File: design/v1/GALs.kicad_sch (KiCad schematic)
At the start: 19 parts, among them IC2 ATF22V10C, IC3 ATF22V10C, IC5 ATF22V10C, IC6 ATF22V10C, IC7 74LS148, IC8 ATF16V8BQL, J9 Conn_02x05_Odd_Even, U5 ATF1504

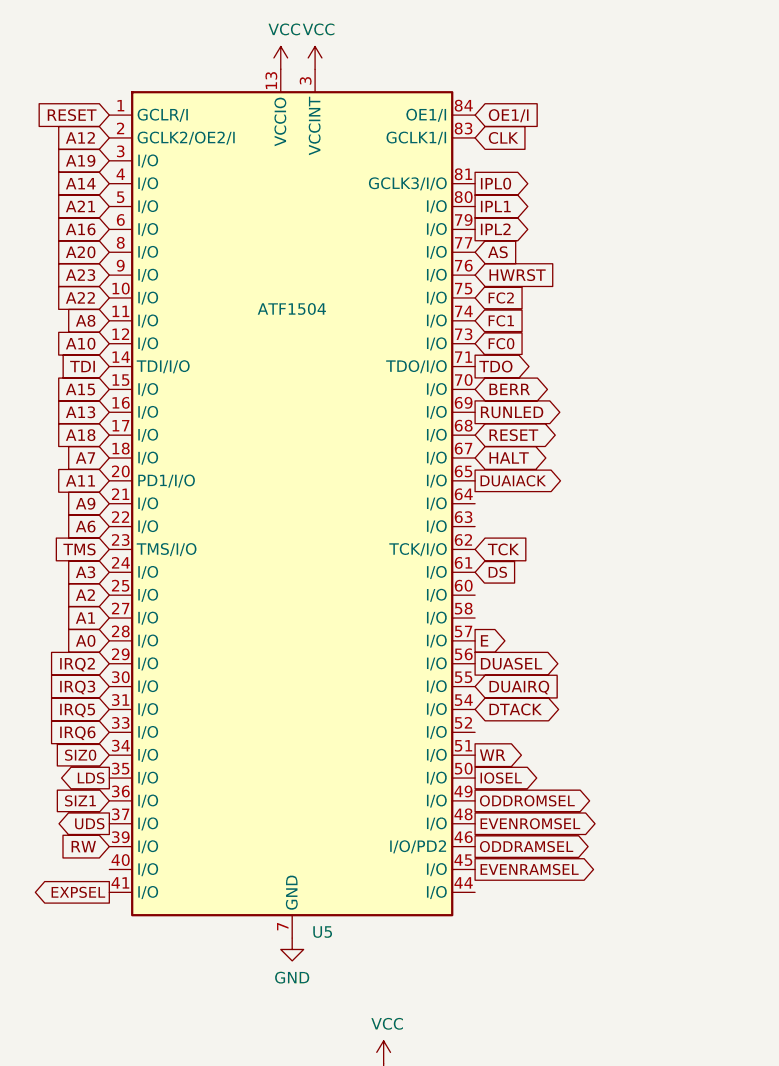
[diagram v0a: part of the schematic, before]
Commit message: Initial pin fit
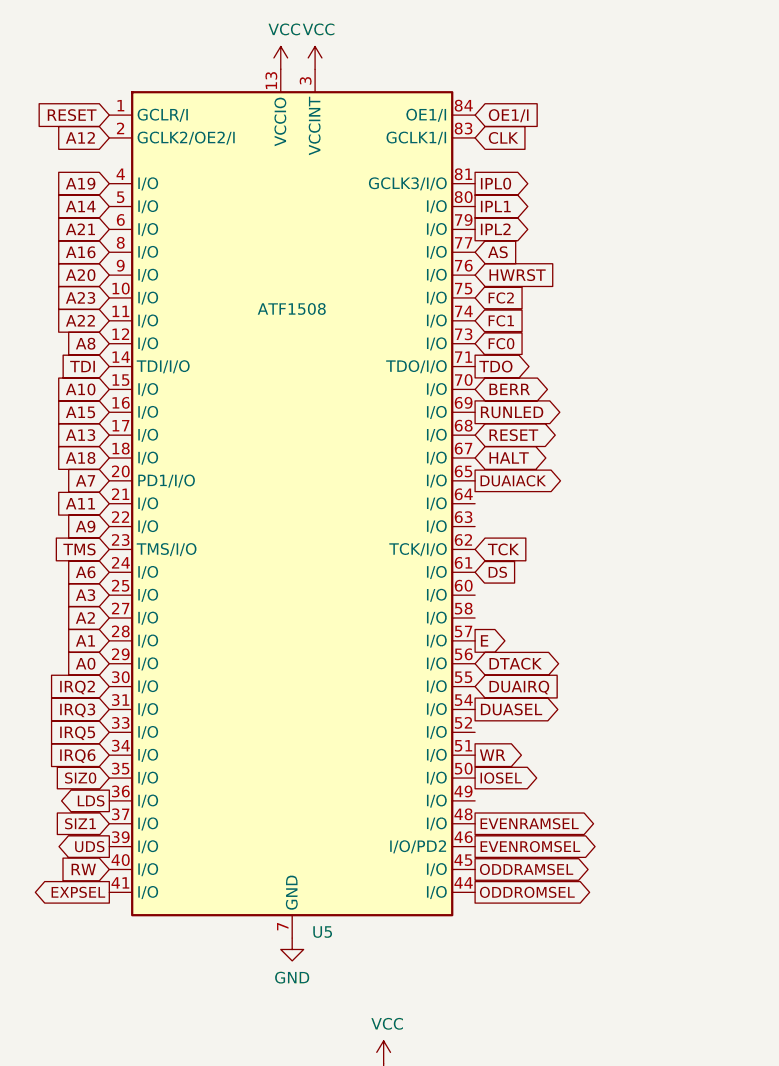
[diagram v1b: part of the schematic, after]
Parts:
- U5: value ATF1504 -> ATF1508
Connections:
- net A0: now also U5.29 (I/O); no longer U5.28 (I/O)
- net A1: now also U5.28 (I/O); no longer U5.27 (I/O)
- net A10: now also U5.15 (I/O); no longer U5.12 (I/O)
- net A11: now also U5.21 (I/O); no longer U5.20 (PD1/I/O)
- net A13: now also U5.17 (I/O); no longer U5.16 (I/O)
- net A14: now also U5.5 (I/O); no longer U5.4 (I/O)
- net A15: now also U5.16 (I/O); no longer U5.15 (I/O)
- net A16: now also U5.8 (I/O); no longer U5.6 (I/O)
- net A18: now also U5.18 (I/O); no longer U5.17 (I/O)
- net A19: now also U5.4 (I/O); no longer U5.3 (VCCINT)
- net A2: now also U5.27 (I/O); no longer U5.25 (I/O)
- net A20: now also U5.9 (I/O); no longer U5.8 (I/O)
- net A21: now also U5.6 (I/O); no longer U5.5 (I/O)
- net A22: now also U5.11 (I/O); no longer U5.10 (I/O)
- net A23: now also U5.10 (I/O); no longer U5.9 (I/O)
- net A3: now also U5.25 (I/O); no longer U5.24 (I/O)
- net A6: now also U5.24 (I/O); no longer U5.22 (I/O)
- net A7: now also U5.20 (PD1/I/O); no longer U5.18 (I/O)
- net A8: now also U5.12 (I/O); no longer U5.11 (I/O)
- net A9: now also U5.22 (I/O); no longer U5.21 (I/O)
- net DTACK: now also U5.56 (I/O); no longer U5.54 (I/O)
- net DUASEL: now also U5.54 (I/O); no longer U5.56 (I/O)
- net EVENRAMSEL: now also U5.48 (I/O); no longer U5.45 (I/O)
- net EVENROMSEL: now also U5.46 (I/O/PD2); no longer U5.48 (I/O)
- net IRQ2: now also U5.30 (I/O); no longer U5.29 (I/O)
- net IRQ3: now also U5.31 (I/O); no longer U5.30 (I/O)
- net IRQ5: now also U5.33 (I/O); no longer U5.31 (I/O)
- net IRQ6: now also U5.34 (I/O); no longer U5.33 (I/O)
- net LDS: now also U5.36 (I/O); no longer U5.35 (I/O)
- net ODDRAMSEL: now also U5.45 (I/O); no longer U5.46 (I/O/PD2)
- net ODDROMSEL: now also U5.44 (I/O); no longer U5.49 (I/O)
- net RW: now also U5.40 (I/O); no longer U5.39 (I/O)
- net SIZ0: now also U5.35 (I/O); no longer U5.34 (I/O)
- net SIZ1: now also U5.37 (I/O); no longer U5.36 (I/O)
- net UDS: now also U5.39 (I/O); no longer U5.37 (I/O)

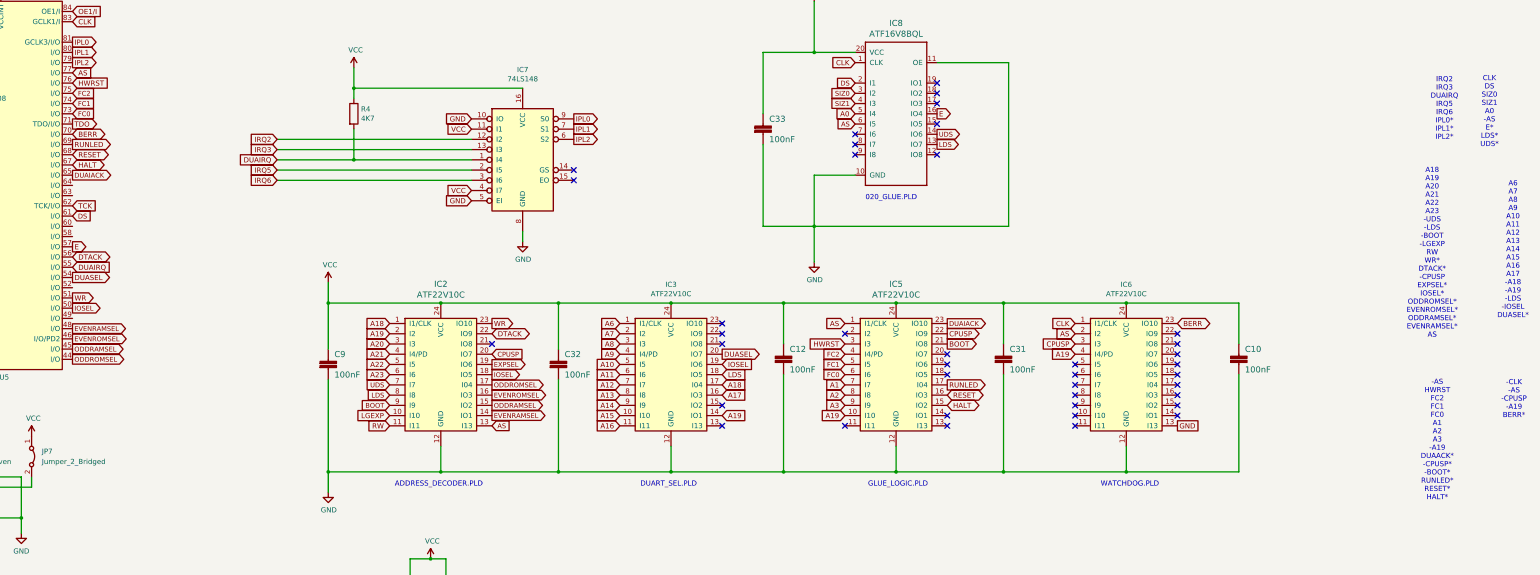
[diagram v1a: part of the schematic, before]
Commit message: Tidy up readme
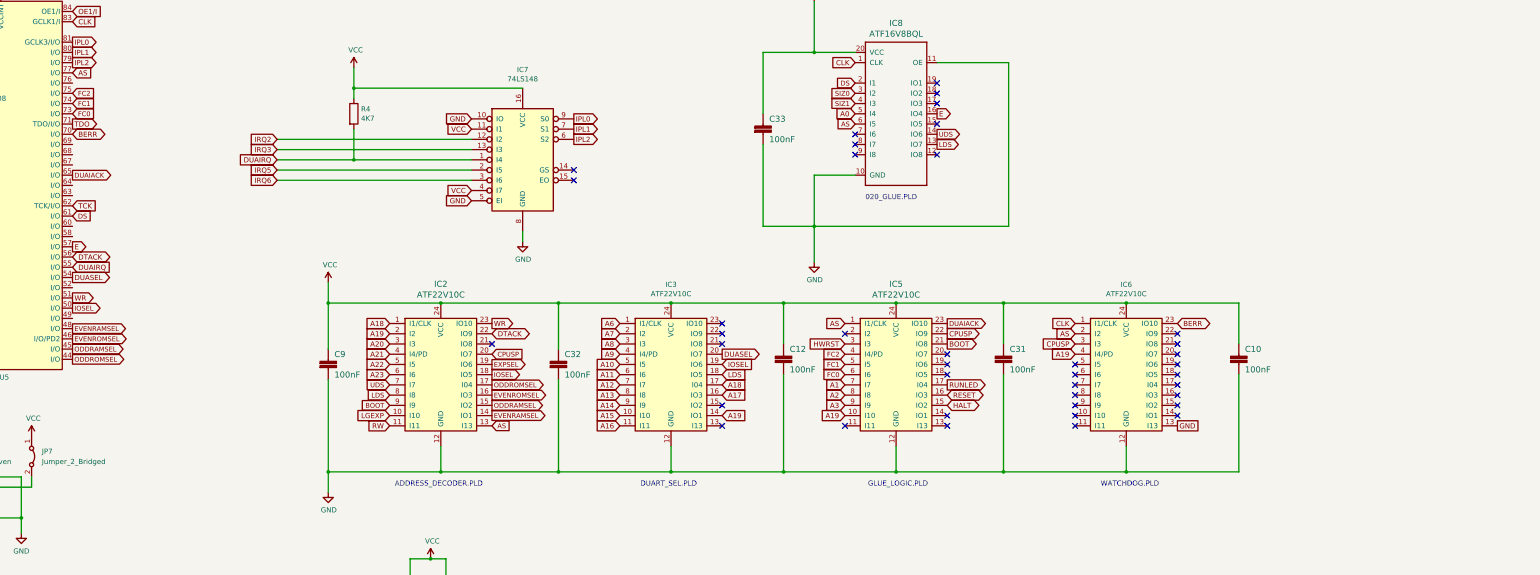
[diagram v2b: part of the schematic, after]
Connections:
- net HALT: no longer U5.67 (I/O)
- net HWRST: no longer U5.76 (I/O)
- net RESET: no longer U5.68 (I/O)
- net RUNLED: no longer U5.69 (I/O)
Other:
- note removed: "-AS HWRST FC2 FC1 FC0 A1 A2 A3 -A19 DUAACK* -CPUSP* -BOOT* RUNLED* RESET* HALT*"
- note removed: "-CLK -AS -CPUSP -A19 BERR*"
- note removed: "A18 A19 A20 A21 A22 A23 -UDS -LDS -BOOT -LGEXP RW WR* DTACK* -CPUSP EXPSEL* IOSEL* ODDROMSEL* EVENROMSEL* ODDRAMSEL* EVENRAMSEL* AS"
- note removed: "A6 A7 A8 A9 A10 A11 A12 A13 A14 A15 A16 A17 -A18 -A19 -LDS -IOSEL DUASEL*"
- note removed: "CLK DS SIZ0 SIZ1 A0 -AS E* LDS* UDS*"
- note removed: "IRQ2 IRQ3 DUAIRQ IRQ5 IRQ6 IPL0* IPL1* IPL2*"
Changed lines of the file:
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@@
-		)
-	)
-	(text "A6\nA7\nA8\nA9\nA10\nA11\nA12\nA13\nA14\nA15\nA16\nA17\n-A18\n-A19\n-LDS\n-IOSEL\nDUASEL*"
-		(exclude_from_sim no)
-		(at 329.692 68.072 0)
-		(effects
-			(font
-				(size 1.27 1.27)
-			)
 		)
 	)
@@
 		)
 	)
-	(text "-CLK\n-AS\n-CPUSP\n-A19\nBERR*\n"
-		(exclude_from_sim no)
-		(at 329.946 105.156 0)
-		(effects
-			(font
-				(size 1.27 1.27)
-			)
-		)
-	)
 	(text "ADDRESS_DECODER.PLD"
 		(exclude_from_sim no)
@@
 		)
 	)
-	(text "IRQ2\nIRQ3\nDUAIRQ\nIRQ5\nIRQ6\nIPL0*\nIPL1*\nIPL2*"
-		(exclude_from_sim no)
-		(at 312.674 33.02 0)
-		(effects
-			(font
-				(size 1.27 1.27)
-			)
-		)
-	)
 	(text "DUART_SEL.PLD"
 		(exclude_from_sim no)
@@
 		)
 	)
-	(text "-AS\nHWRST\nFC2\nFC1\nFC0\nA1\nA2\nA3\n-A19\nDUAACK*\n-CPUSP*\n-BOOT*\nRUNLED*\nRESET*\nHALT*"
-		(exclude_from_sim no)
-		(at 310.896 115.316 0)
-		(effects
-			(font
-				(size 1.27 1.27)
-			)
-		)
-	)
-	(text "CLK\nDS\nSIZ0\nSIZ1\nA0\n-AS\nE*\nLDS*\nUDS*"
-		(exclude_from_sim no)
-		(at 323.85 33.782 0)
-		(effects
-			(font
-				(size 1.27 1.27)
-			)
-		)
-	)
-	(text "A18\nA19\nA20\nA21\nA22\nA23\n-UDS\n-LDS\n-BOOT\n-LGEXP\nRW\nWR*\nDTACK*\n-CPUSP\nEXPSEL*\nIOSEL*\nODDROMSEL*\nEVENROMSEL*\nODDRAMSEL*\nEVENRAMSEL*\nAS"
-		(exclude_from_sim no)
-		(at 309.626 68.834 0)
-		(effects
-			(font
-				(size 1.27 1.27)
-			)
-		)
-	)
 	(text "WATCHDOG.PLD"
 		(exclude_from_sim no)
@@
 		)
 	)
-	(global_label "RUNLED"
-		(shape output)
-		(at -27.94 41.91 0)
-		(fields_autoplaced yes)
-		(effects
-			(font
-				(size 1.27 1.27)
-			)
-			(justify left)
-		)
-		(property "Intersheetrefs" "${INTERSHEET_REFS}"
-			(at -217.17 -59.69 0)
-			(effects
-				(font
-					(size 1.27 1.27)
-				)
-				(hide yes)
-			)
-		)
-	)
 	(global_label "DS"
 		(shape input)
@@
 		)
 	)
-	(global_label "RESET"
-		(shape tri_state)
-		(at -27.94 44.45 0)
-		(fields_autoplaced yes)
-		(effects
-			(font
-				(size 1.27 1.27)
-			)
-			(justify left)
-		)
-		(property "Intersheetrefs" "${INTERSHEET_REFS}"
-			(at -217.17 -59.69 0)
-			(effects
-				(font
-					(size 1.27 1.27)
-				)
-				(hide yes)
-			)
-		)
-	)
 	(global_label "IPL0"
 		(shape output)
@@
 		)
 	)
-	(global_label "HALT"
-		(shape tri_state)
-		(at -27.94 46.99 0)
-		(fields_autoplaced yes)
-		(effects
-			(font
-				(size 1.27 1.27)
-			)
-			(justify left)
-		)
-		(property "Intersheetrefs" "${INTERSHEET_REFS}"
-			(at -217.17 -59.69 0)
-			(effects
-				(font
-					(size 1.27 1.27)
-				)
-				(hide yes)
-			)
-		)
-	)
 	(global_label "A15"
 		(shape input)
@@
 			(effects
 				(font
-					(size 1.27 1.27)
-				)
-				(hide yes)
-			)
-		)
-	)
-	(global_label "HWRST"
-		(shape input)
-		(at -27.94 26.67 0)
-		(fields_autoplaced yes)
-		(effects
-			(font
-				(size 1.27 1.27)
-			)
-			(justify left)
-		)
-		(property "Intersheetrefs" "${INTERSHEET_REFS}"
-			(at 135.89 -64.77 0)
-			(effects
-				(font
